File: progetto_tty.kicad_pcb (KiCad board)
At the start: 2 copper layers, 56 parts, among them J1 Conn_02x05_Odd_Even, J2 Conn_Coaxial_Power, Q1 BC548, Q10 IRF9540N, Q11 IRF540N, Q12 BC548, Q2 IRF9540N, Q3 IRF540N, Q4 IRF9540N, Q5 IRF540N, Q6 BC548, Q7 BC548, Q8 IRF9540N, Q9 IRF540N, U1 ATmega328P-P, U2 L7805, Y1 16MHz

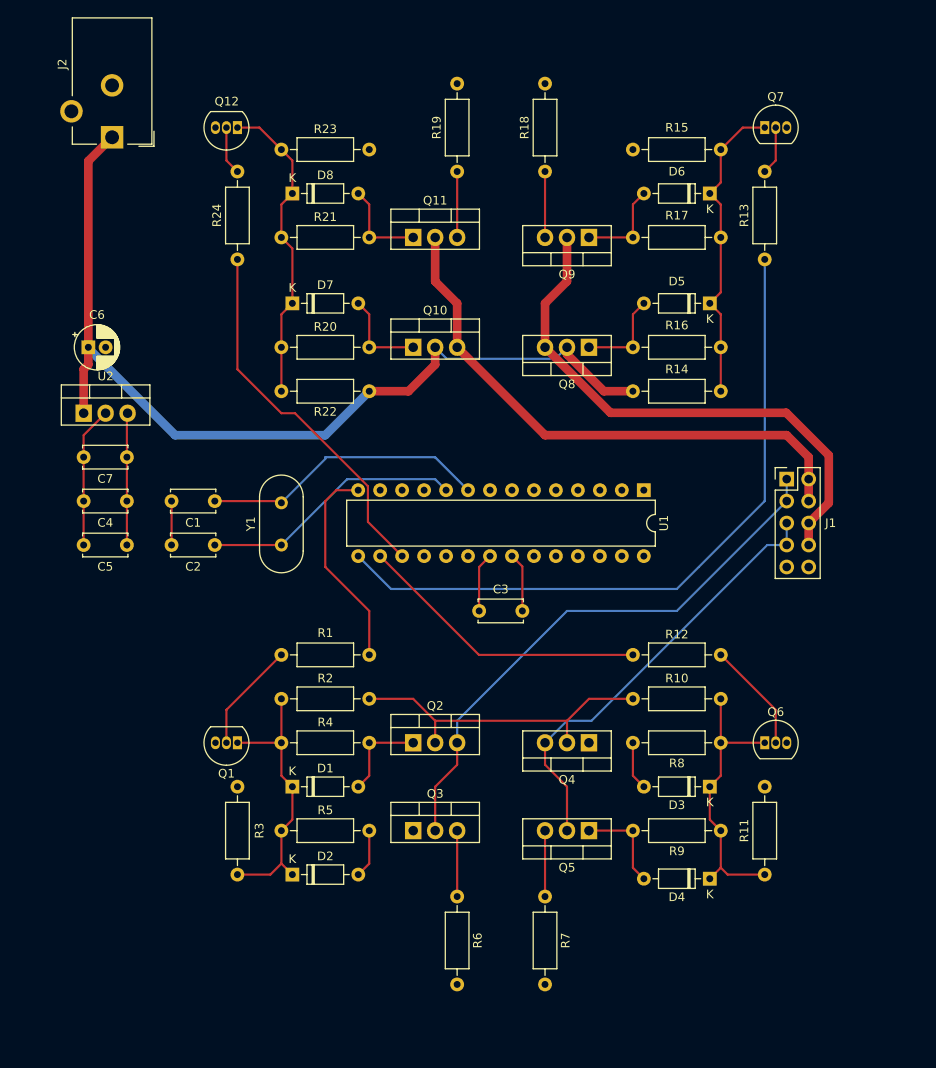
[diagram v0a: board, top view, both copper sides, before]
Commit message: pcb
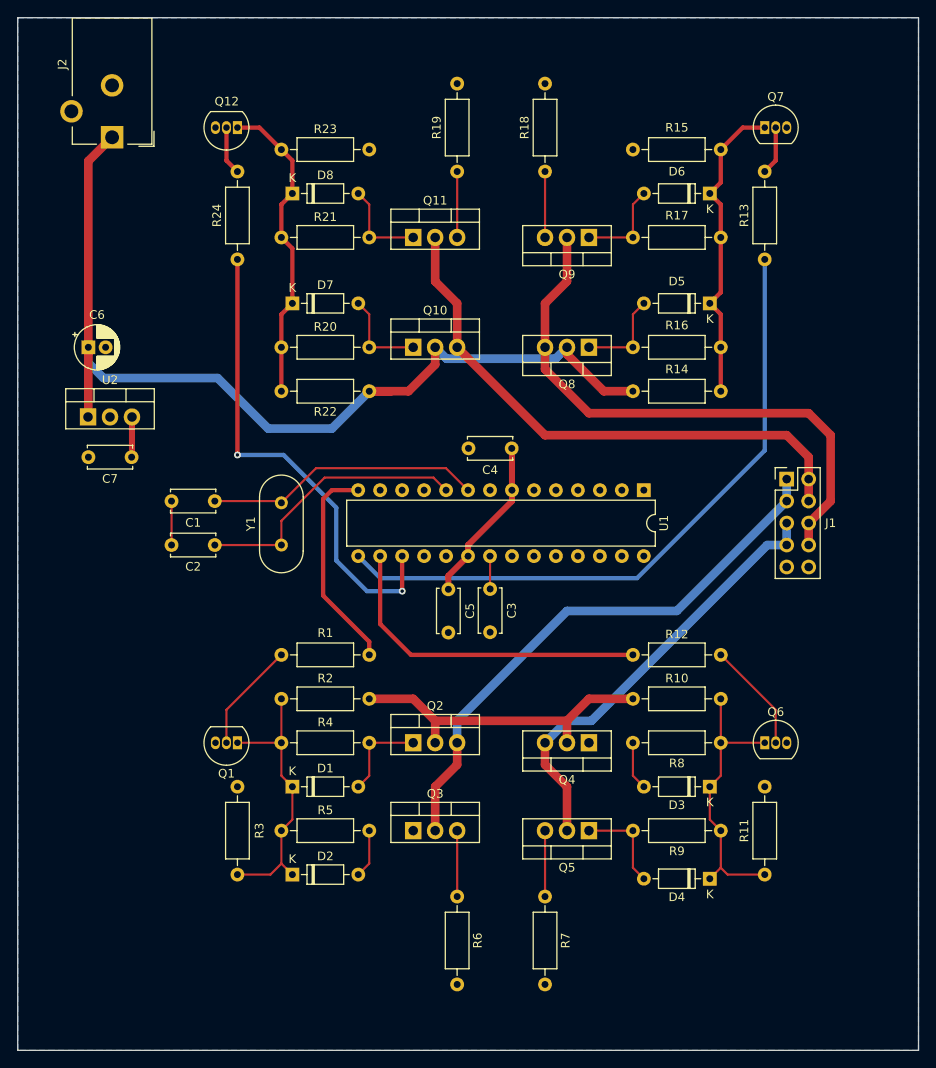
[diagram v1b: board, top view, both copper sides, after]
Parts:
- moved C4 44.9 mm to (123.2, 72.6)
- moved C5 37.5 mm to (115.8, 88.9), turned to -90 degrees
- moved C3 2.84 mm to (120.7, 88.9), turned to -90 degrees
- moved U2 0.67 mm to (74.2, 69.0)
- moved C7 0.55 mm to (79.2, 73.7)
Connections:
- J1 pad 2: GREY_2 -> +12V
- J1 pad 4: GREY_2 -> +12V
- J1 pad 6: BLACK_2 -> +12V
- J1 pad 8: BLACK_2 -> +12V
- Q10 pad 3: GREY_2 -> +12V
- Q11 pad 2: GREY_2 -> +12V
- Q8 pad 3: BLACK_2 -> +12V
- Q9 pad 2: BLACK_2 -> +12V
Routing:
- net +12V: track 149.8 -> 281.3 mm
- net GREY_2: track 64.7 -> 0.00 mm
- net BLACK_2: track 63.1 -> 0.00 mm
- net GND: track 28.2 -> 5.11 mm
- net /D11: track 43.1 -> 55.8 mm, vias 0 -> 2
- net +5V: track 15.3 -> 24.0 mm
- net /D10: track 34.0 -> 38.6 mm
- net /D9: track 80.7 -> 76.3 mm
- net Net-(C3-Pad1): track 6.86 -> 3.80 mm
- net Net-(C2-Pad1): track 30.4 -> 32.2 mm
- net Net-(C1-Pad1): track 33.6 -> 32.4 mm
- net /D8: track 24.2 -> 24.7 mm
- added copper zone on B.Cu, net GND
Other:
- board outline added: 104.1 x 119.4 mm
